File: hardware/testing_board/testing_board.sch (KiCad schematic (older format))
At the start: 40 parts

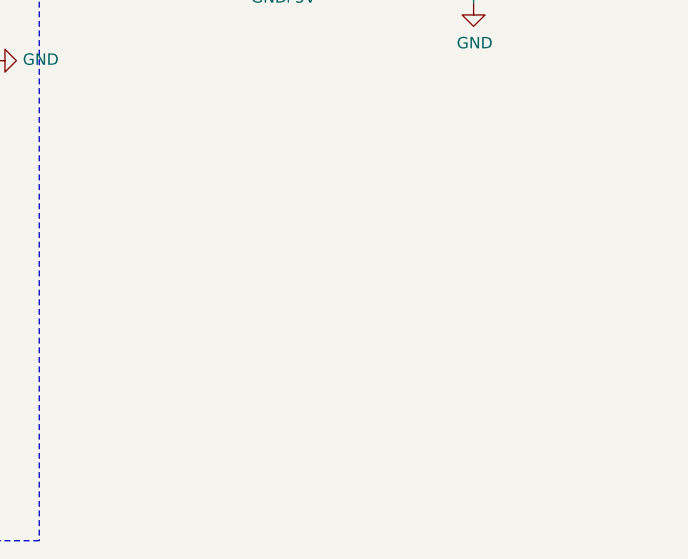
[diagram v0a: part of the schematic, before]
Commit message: updates to training board
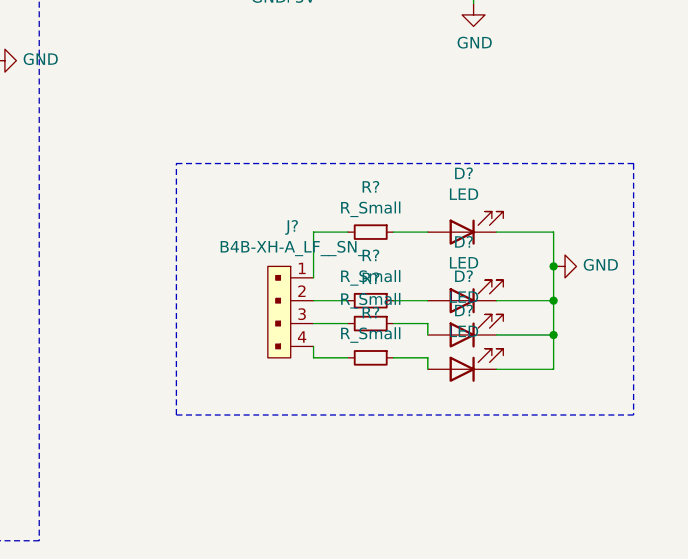
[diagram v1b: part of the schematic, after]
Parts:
- added D? (x4): LED, symbol Device:LED
- added J?: B4B-XH-A_LF__SN_, digikey-footprints:PinHeader_1x4_P2.5mm_Drill1.1mm, symbol dk_Rectangular-Connectors-Headers-Male-Pins:B4B-XH-A_LF__SN_
- added R? (x4): R_Small, symbol Device:R_Small
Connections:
- net GND: now also D?.1 (K), D?.1 (K), D?.1 (K), D?.1 (K)
- new net: J?.1, R?.2
- new net: J?.2, R?.2
- new net: J?.3, R?.2
- new net: J?.4, R?.2
- new net: D?.2 (A), R?.1 (x4)
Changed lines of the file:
@@
 Wire Notes Line
 	5500 2200 5500 1100
+$Comp
+L dk_Rectangular-Connectors-Headers-Male-Pins:B4B-XH-A_LF__SN_ J?
+U 1 1 6164C117
+P 6050 5750
+F 0 "J?" V 5825 5758 50  0000 C CNN
+F 1 "B4B-XH-A_LF__SN_" V 5916 5758 50  0000 C CNN
+F 2 "digikey-footprints:PinHeader_1x4_P2.5mm_Drill1.1mm" H 6250 5950 60  0001 L CNN
+F 3 "http://www.jst-mfg.com/product/pdf/eng/eXH.pdf" H 6250 6050 60  0001 L CNN
+F 4 "455-2249-ND" H 6250 6150 60  0001 L CNN "Digi-Key_PN"
+F 5 "B4B-XH-A(LF)(SN)" H 6250 6250 60  0001 L CNN "MPN"
+F 6 "Connectors, Interconnects" H 6250 6350 60  0001 L CNN "Category"
+F 7 "Rectangular Connectors - Headers, Male Pins" H 6250 6450 60  0001 L CNN "Family"
+F 8 "http://www.jst-mfg.com/product/pdf/eng/eXH.pdf" H 6250 6550 60  0001 L CNN "DK_Datasheet_Link"
+F 9 "/product-detail/en/jst-sales-america-inc/B4B-XH-A(LF)(SN)/455-2249-ND/1651047" H 6250 6650 60  0001 L CNN "DK_Detail_Page"
+F 10 "CONN HEADER VERT 4POS 2.5MM" H 6250 6750 60  0001 L CNN "Description"
+F 11 "JST Sales America Inc." H 6250 6850 60  0001 L CNN "Manufacturer"
+F 12 "Active" H 6250 6950 60  0001 L CNN "Status"
+	1    6050 5750
+	0    1    1    0
+$EndComp
+$Comp
+L Device:R_Small R?
+U 1 1 6164C11F
+P 6400 5850
+F 0 "R?" V 6204 5850 50  0000 C CNN
+F 1 "R_Small" V 6295 5850 50  0000 C CNN
+F 2 "" H 6400 5850 50  0001 C CNN
+F 3 "~" H 6400 5850 50  0001 C CNN
+	1    6400 5850
+	0    1    1    0
+$EndComp
+$Comp
+L Device:R_Small R?
+U 1 1 6164C125
+P 6400 5550
+F 0 "R?" V 6204 5550 50  0000 C CNN
+F 1 "R_Small" V 6295 5550 50  0000 C CNN
+F 2 "" H 6400 5550 50  0001 C CNN
+F 3 "~" H 6400 5550 50  0001 C CNN
+	1    6400 5550
+	0    1    1    0
+$EndComp
+$Comp
+L Device:LED D?
+U 1 1 6164C12B
+P 6800 5850
+F 0 "D?" H 6793 5595 50  0000 C CNN
+F 1 "LED" H 6793 5686 50  0000 C CNN
+F 2 "" H 6800 5850 50  0001 C CNN
+F 3 "~" H 6800 5850 50  0001 C CNN
+	1    6800 5850
+	-1   0    0    1
+$EndComp
+$Comp
+L Device:LED D?
+U 1 1 6164C131
+P 6800 5550
+F 0 "D?" H 6793 5295 50  0000 C CNN
+F 1 "LED" H 6793 5386 50  0000 C CNN
+F 2 "" H 6800 5550 50  0001 C CNN
+F 3 "~" H 6800 5550 50  0001 C CNN
+	1    6800 5550
+	-1   0    0    1
+$EndComp
+Wire Wire Line
+	6150 5750 6150 5550
+Wire Wire Line
+	6150 5550 6300 5550
+Wire Wire Line
+	6500 5550 6650 5550
+Wire Wire Line
+	6150 5850 6300 5850
+Wire Wire Line
+	6500 5850 6650 5850
+$Comp
+L power:GND #PWR?
+U 1 1 6164C13C
+P 7200 5700
+F 0 "#PWR?" H 7200 5450 50  0001 C CNN
+F 1 "GND" V 7205 5572 50  0000 R CNN
+F 2 "" H 7200 5700 50  0001 C CNN
+F 3 "" H 7200 5700 50  0001 C CNN
+	1    7200 5700
+	0    -1   -1   0
+$EndComp
+Wire Wire Line
+	6950 5550 7200 5550
+Wire Wire Line
+	7200 5550 7200 5700
+Wire Wire Line
+	6950 5850 7200 5850
+Wire Wire Line
+	7200 5850 7200 5700
+Connection ~ 7200 5700
+$Comp
+L Device:R_Small R?
+U 1 1 61668427
+P 6400 5950
+F 0 "R?" V 6204 5950 50  0000 C CNN
+F 1 "R_Small" V 6295 5950 50  0000 C CNN
+F 2 "" H 6400 5950 50  0001 C CNN
+F 3 "~" H 6400 5950 50  0001 C CNN
+	1    6400 5950
+	0    1    1    0
+$EndComp
+$Comp
+L Device:R_Small R?
+U 1 1 616689D9
+P 6400 6100
+F 0 "R?" V 6204 6100 50  0000 C CNN
+F 1 "R_Small" V 6295 6100 50  0000 C CNN
+F 2 "" H 6400 6100 50  0001 C CNN
+F 3 "~" H 6400 6100 50  0001 C CNN
+	1    6400 6100
+	0    1    1    0
+$EndComp
+$Comp
+L Device:LED D?
+U 1 1 61668C6A
+P 6800 6000
+F 0 "D?" H 6793 5745 50  0000 C CNN
+F 1 "LED" H 6793 5836 50  0000 C CNN
+F 2 "" H 6800 6000 50  0001 C CNN
+F 3 "~" H 6800 6000 50  0001 C CNN
+	1    6800 6000
+	-1   0    0    1
+$EndComp
+$Comp
+L Device:LED D?
+U 1 1 6166925E
+P 6800 6150
+F 0 "D?" H 6793 5895 50  0000 C CNN
+F 1 "LED" H 6793 5986 50  0000 C CNN
+F 2 "" H 6800 6150 50  0001 C CNN
+F 3 "~" H 6800 6150 50  0001 C CNN
+	1    6800 6150
+	-1   0    0    1
+$EndComp
+Wire Wire Line
+	6150 5950 6300 5950
+Wire Wire Line
+	6150 6050 6150 6100
+Wire Wire Line
+	6150 6100 6300 6100
+Wire Wire Line
+	6500 5950 6650 5950
+Wire Wire Line
+	6650 5950 6650 6000
+Wire Wire Line
+	6500 6100 6650 6100
+Wire Wire Line
+	6650 6100 6650 6150
+Wire Wire Line
+	6950 6000 7200 6000
+Wire Wire Line
+	7200 6000 7200 5850
+Connection ~ 7200 5850
+Wire Wire Line
+	6950 6150 7200 6150
+Wire Wire Line
+	7200 6150 7200 6000
+Connection ~ 7200 6000
+Wire Notes Line
+	5550 5250 7550 5250
+Wire Notes Line
+	7550 5250 7550 6350
+Wire Notes Line
+	7550 6350 5550 6350
+Wire Notes Line
+	5550 6350 5550 5250
 $EndSCHEMATC
